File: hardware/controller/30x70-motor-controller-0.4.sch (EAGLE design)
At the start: 19 parts, among them IC1 TS432A-A3G, IC2 TS432A-A3G

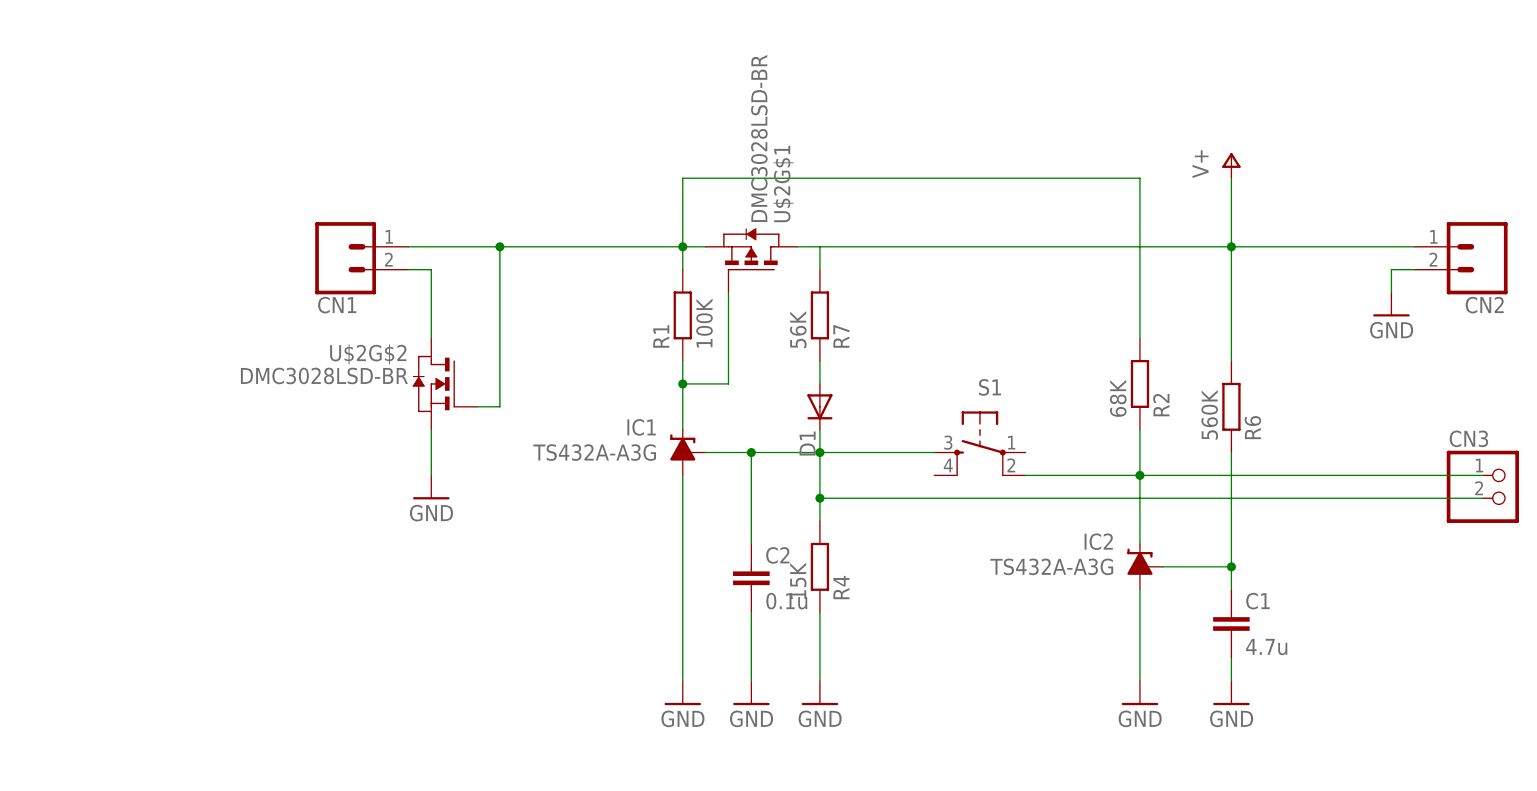
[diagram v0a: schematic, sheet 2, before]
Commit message: Lots of controller designs
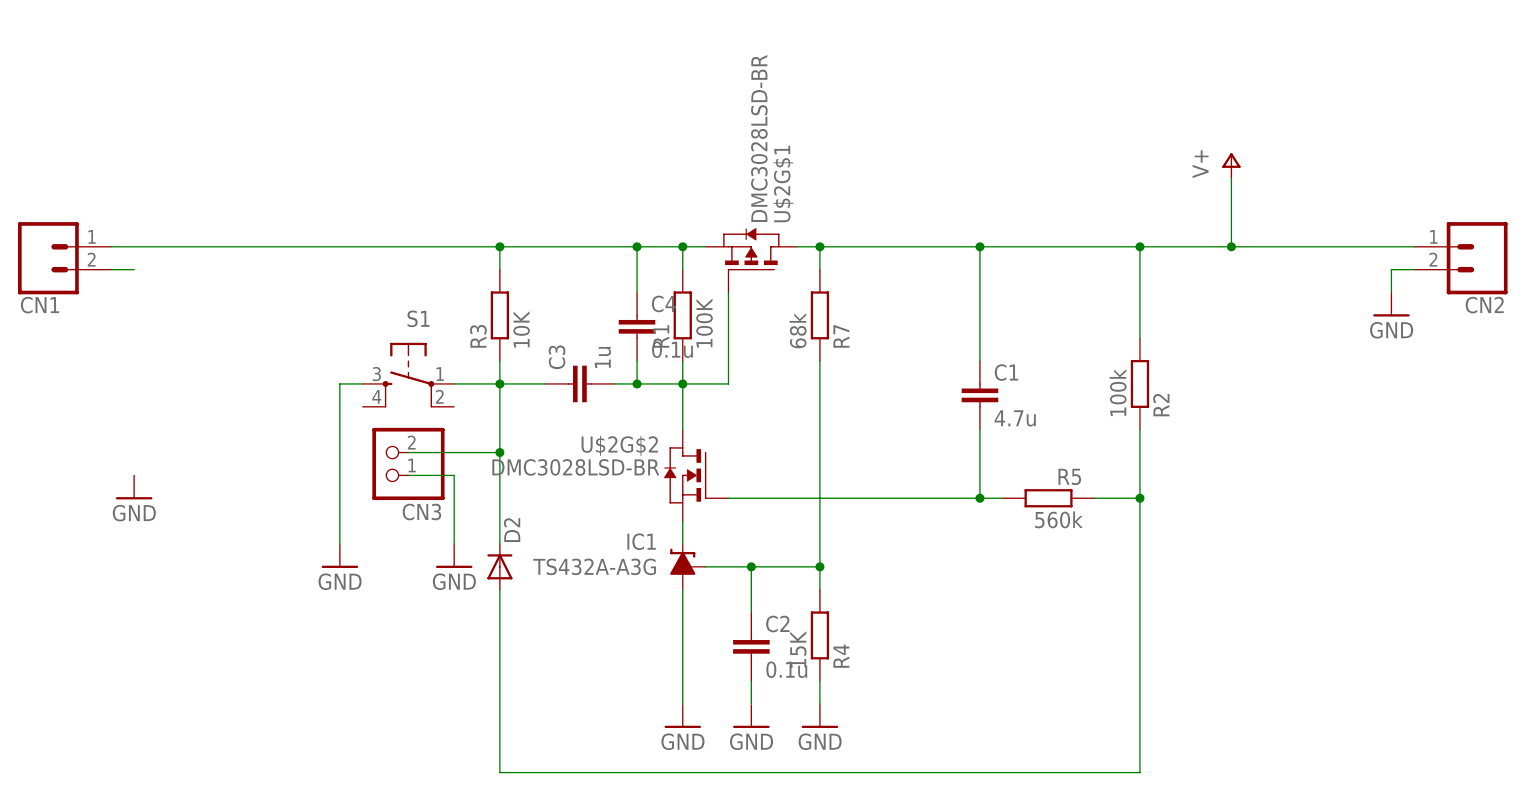
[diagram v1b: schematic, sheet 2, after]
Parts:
- removed D1: (no value), diode:DIODE-D-2.5
- removed IC2: TS432A-A3G, assorted:TS432A-A3G
- removed R6: 560K, resistor:R-EU_0204/2V
- added C3: 1u, resistor:C-EU025-024X044
- added C4: 0.1u, resistor:C-EU025-024X044
- added D2: (no value), diode:DIODE-D-2.5
- added R3: 10K, resistor:R-EU_0204/2V
- added R5: 560k, resistor:R-EU_0204/7
- C1: device resistor:C-EU050-024X044 -> resistor:C-EU025-025X050
- R2: value 68K -> 100k; device resistor:R-EU_0207/15 -> resistor:R-EU_0204/2V
- R7: value 56K -> 68k
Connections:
- new net N$17: C3.1, CN3.2, D2.C, R3.1, S1.P
- net GND: now also CN3.1, S1.S; no longer C1.2, IC2.A, U$2G$2.S
- net N$10: now also D2.A, R2.1, R5.1; no longer C1.1, IC2.FB, R6.1
- net N$13: now also IC1.C, U$2G$2.S; no longer D1.A, R7.1
- net N$5: now also C4.1, R3.2; no longer R2.2, U$2G$2.G
- net N$6: now also C3.2, C4.2, U$2G$2.D; no longer IC1.C
- net N$7: no longer U$2G$2.D
- net N$8: now also R7.1; no longer CN3.2, D1.C, S1.S
- net N$9: now also C1.2, R5.2, U$2G$2.G; no longer CN3.1, IC2.C, R2.1, S1.P1
- net V+: now also C1.1, R2.2; no longer R6.2
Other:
- moved on the sheet: C1, C2, CN1, CN3, IC1, R4, S1, U$2G$2
